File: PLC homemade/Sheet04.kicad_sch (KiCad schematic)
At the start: 9 parts, among them IC1 PCF8574DGVR, J2 1803316

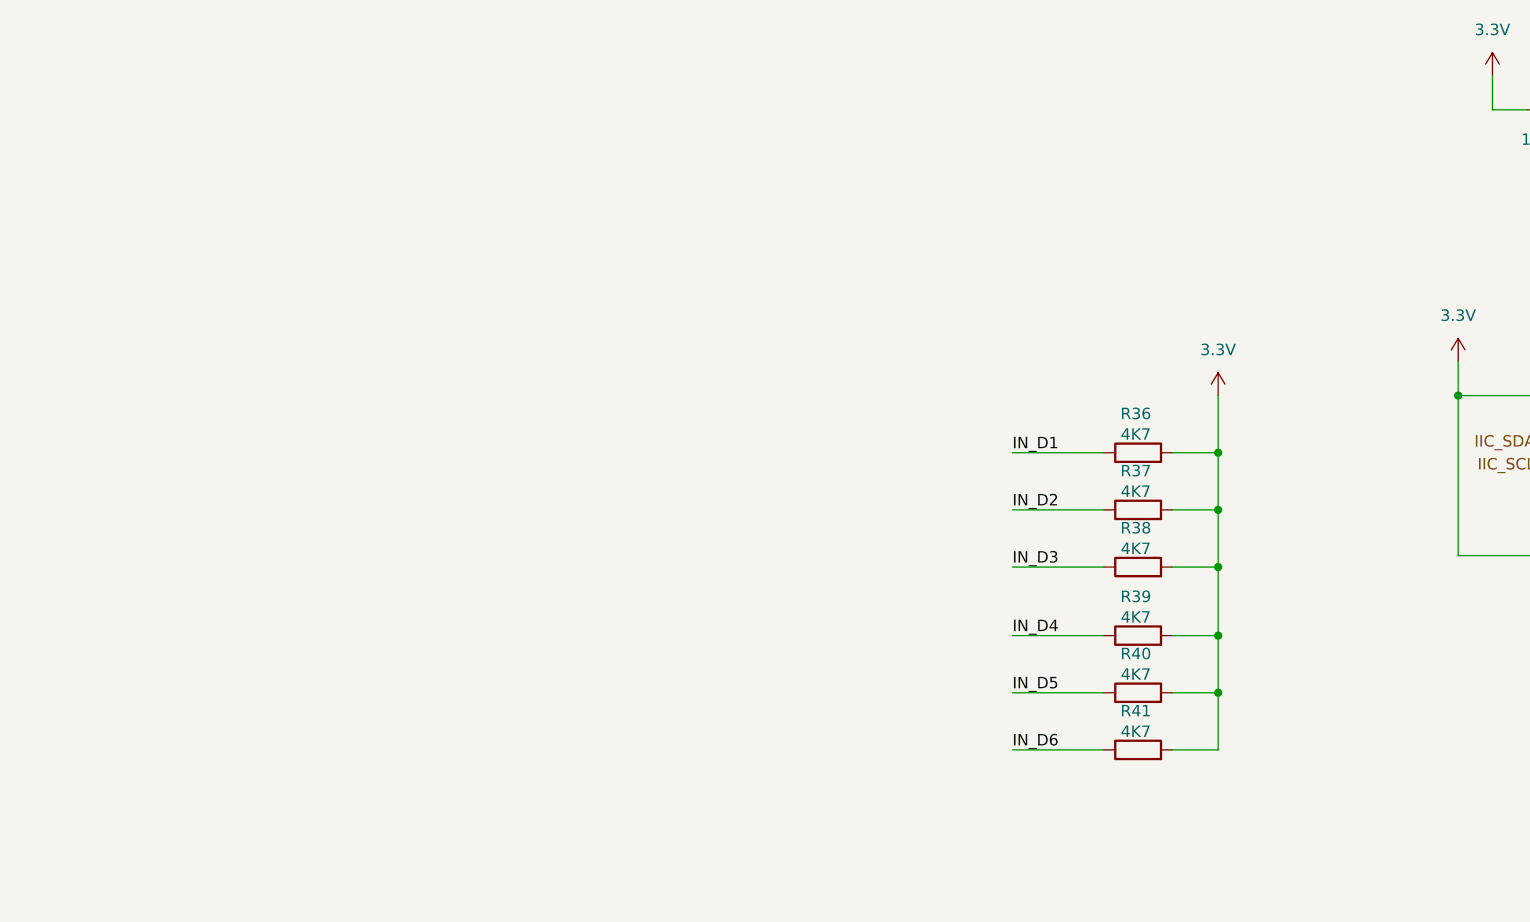
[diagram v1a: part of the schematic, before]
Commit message: :art: COMPLETED SHEET4
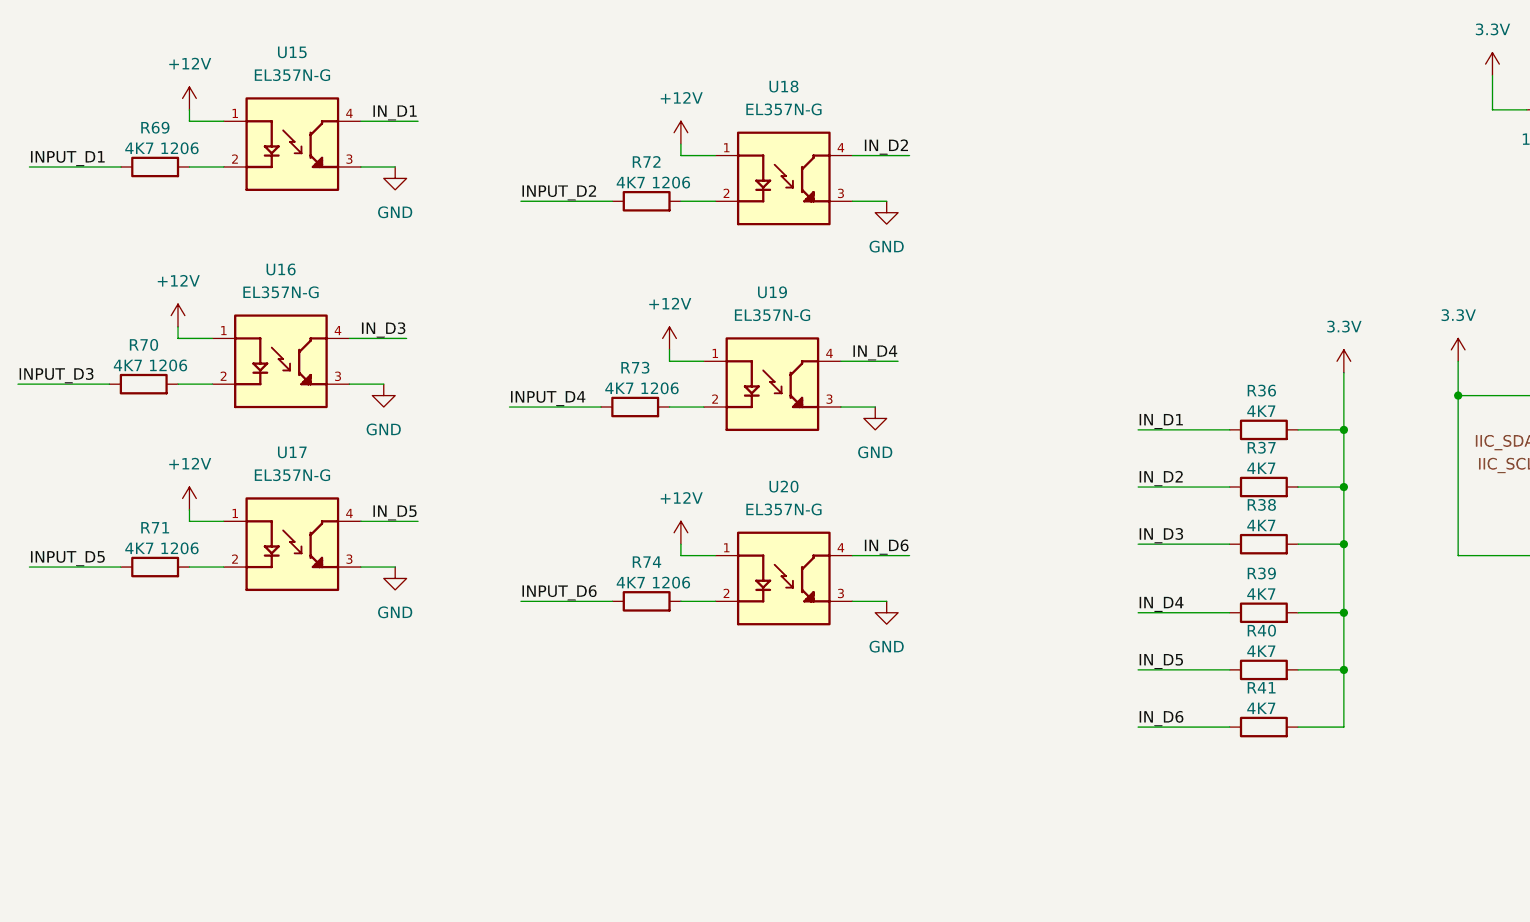
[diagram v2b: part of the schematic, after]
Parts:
- added R69, R70, R71, R72, R73, R74: 4K7 1206, symbol Device:R
- added U15, U16, U17, U18, U19, U20: EL357N-G, EL357N-G:OPTO_EL357N-G, symbol EL357N-G:EL357N-G
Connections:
- net GND: now also U15.3, U16.3, U17.3, U18.3, U19.3, U20.3
- net INPUT_D1: now also R69.1
- net INPUT_D2: now also R72.1
- net INPUT_D3: now also R70.1
- net INPUT_D4: now also R73.1
- net INPUT_D5: now also R71.1
- net INPUT_D6: now also R74.1
- net IN_D1: now also U15.4
- net IN_D2: now also U18.4
- net IN_D3: now also U16.4
- net IN_D4: now also U19.4
- net IN_D5: now also U17.4
- net IN_D6: now also U20.4
- new net: R70.2, U16.2
- new net: R71.2, U17.2
- new net: R73.2, U19.2
- new net: R72.2, U18.2
- new net: R69.2, U15.2
- new net: R74.2, U20.2
- new net +12V: U15.1, U16.1, U17.1, U18.1, U19.1, U20.1
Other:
- moved on the sheet: R36, R37, R38, R39, R40, R41

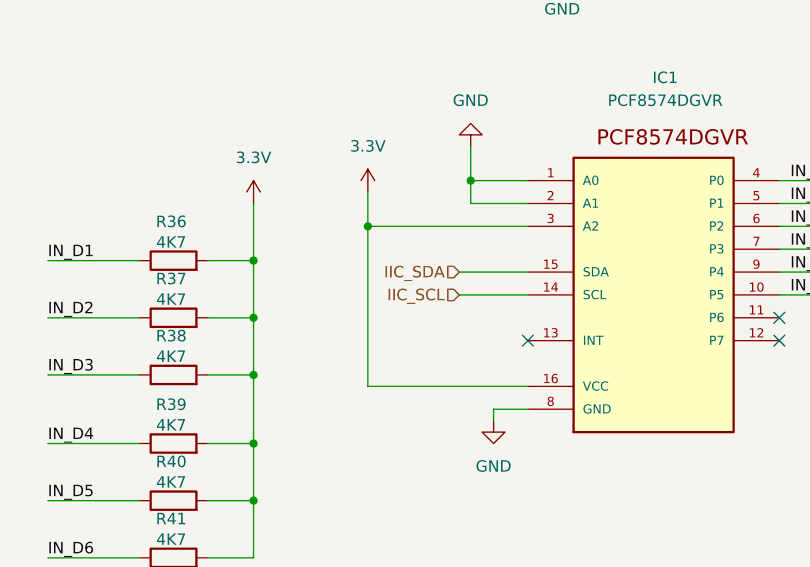
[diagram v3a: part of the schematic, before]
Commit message: :clown_face: changed HEIRACHIAL to global
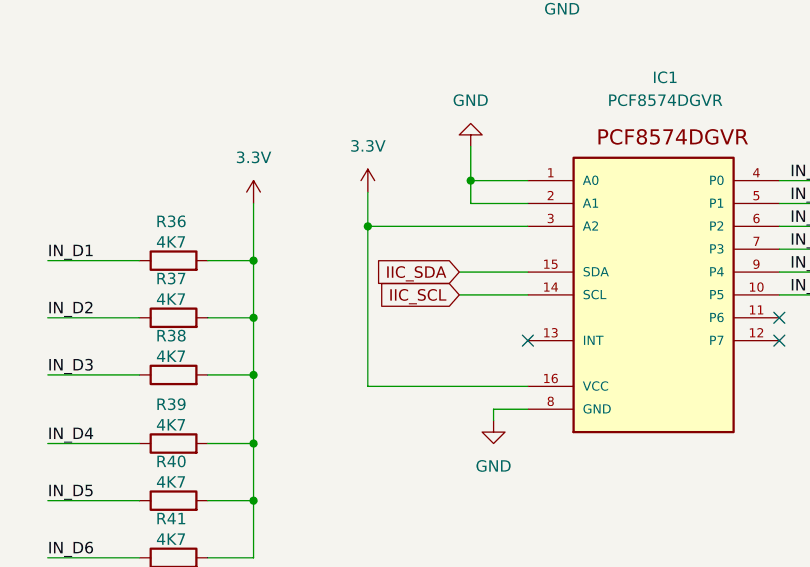
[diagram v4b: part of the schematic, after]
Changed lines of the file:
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@@
 		)
 	)
-	(hierarchical_label "IIC_SCL"
+	(global_label "IIC_SDA"
 		(shape input)
-		(at 185.42 62.23 180)
+		(at 185.42 59.69 180)
+		(fields_autoplaced yes)
 		(effects
 			(font
@@
 			(justify right)
 		)
+		(property "Intersheetrefs" "${INTERSHEET_REFS}"
+			(at 175.4195 59.69 0)
+			(effects
+				(font
+					(size 1.27 1.27)
+				)
+				(justify right)
+				(hide yes)
+			)
+		)
 	)
-	(hierarchical_label "IIC_SDA"
+	(global_label "IIC_SCL"
 		(shape input)
-		(at 185.42 59.69 180)
+		(at 185.42 62.23 180)
+		(fields_autoplaced yes)
 		(effects
 			(font
@@
 			(justify right)
 		)
+		(property "Intersheetrefs" "${INTERSHEET_REFS}"
+			(at 175.48 62.23 0)
+			(effects
+				(font
+					(size 1.27 1.27)
+				)
+				(justify right)
+				(hide yes)
+			)
+		)
 	)

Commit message: :tada: Run Electrical rule checker All errors corrected
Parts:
- C29: footprint (none) -> Capacitor_SMD:C_01005_0402Metric
- R36, R37, R38, R39, R40, R41, R69, R70, R71, R72, R73, R74: footprint (none) -> Resistor_SMD:R_01005_0402Metric
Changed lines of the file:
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@@
 			)
 		)
-		(property "Footprint" ""
+		(property "Footprint" "Resistor_SMD:R_01005_0402Metric"
 			(at 153.67 72.898 90)
 			(effects
@@
 			)
 		)
-		(property "Footprint" ""
+		(property "Footprint" "Capacitor_SMD:C_01005_0402Metric"
 			(at 190.5 21.8948 0)
 			(effects
@@
 			)
 		)
-		(property "Footprint" ""
+		(property "Footprint" "Resistor_SMD:R_01005_0402Metric"
 			(at 153.67 86.868 90)
 			(effects
@@
 			)
 		)
-		(property "Footprint" ""
+		(property "Footprint" "Resistor_SMD:R_01005_0402Metric"
 			(at 29.21 55.118 90)
 			(effects
@@
 			)
 		)
-		(property "Footprint" ""
+		(property "Footprint" "Resistor_SMD:R_01005_0402Metric"
 			(at 153.67 80.518 90)
 			(effects
@@
 			)
 		)
-		(property "Footprint" ""
+		(property "Footprint" "Resistor_SMD:R_01005_0402Metric"
 			(at 153.67 66.548 90)
 			(effects
@@
 			)
 		)
-		(property "Footprint" ""
+		(property "Footprint" "Resistor_SMD:R_01005_0402Metric"
 			(at 85.09 34.798 90)
 			(effects
@@
 			)
 		)
-		(property "Footprint" ""
+		(property "Footprint" "Resistor_SMD:R_01005_0402Metric"
 			(at 153.67 60.198 90)
 			(effects
@@
 			)
 		)
-		(property "Footprint" ""
+		(property "Footprint" "Resistor_SMD:R_01005_0402Metric"
 			(at 30.48 30.988 90)
 			(effects
@@
 			)
 		)
-		(property "Footprint" ""
+		(property "Footprint" "Resistor_SMD:R_01005_0402Metric"
 			(at 83.82 57.658 90)
 			(effects
@@
 			)
 		)
-		(property "Footprint" ""
+		(property "Footprint" "Resistor_SMD:R_01005_0402Metric"
 			(at 85.09 79.248 90)
 			(effects
@@
 			)
 		)
-		(property "Footprint" ""
+		(property "Footprint" "Resistor_SMD:R_01005_0402Metric"
 			(at 153.67 93.218 90)
 			(effects
@@
 			)
 		)
-		(property "Footprint" ""
+		(property "Footprint" "Resistor_SMD:R_01005_0402Metric"
 			(at 30.48 75.438 90)
 			(effects
